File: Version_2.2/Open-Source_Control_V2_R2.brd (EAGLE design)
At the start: 121.9 x 129.5 mm, 344 parts, among them IC10 MCP6002SMT, IC11 MCP6002SMT, IC12 MCP6002SMT, IC14 MCP6002SMT, IC2 ULN2003AD, IC4 74HC165D, IC5 74HC165D, J24 6p-2.54, K1 JS1-24V-F, K2 JS1-24V-F, K3 JS1-24V-F, K4 JS1-24V-F, K5 JS1-24V-F, Q1 MMBT2907, T4 DA2304-AL, U1 OSD3358-512M-ICB, U16 AT97SC3205T-G3M4400B, U2 TPD4S012_DRY_6_P1_M, U27 LAN8710, U28 TCAN1051HV, U29 MAX3483EESA+T, U4 APX811-31UGSOT, U40 ISO3086TDW, U5 TLVH431, U6 SN74LVC2G241_DCU_8, X1 10118194-0001LF, X10 MC4, X11 MC4, X12 MC4, X2 J0011D01BNL, X21 MC10, X24 MSTBA2, X3 MC4, X4 CTI-JTAG, X41 MSTBA3, X5 DM3CS-SF, X6 6p-2.54, X7 TH-2X10, X8 MC4, Y7 7A-25.000MAAE-T

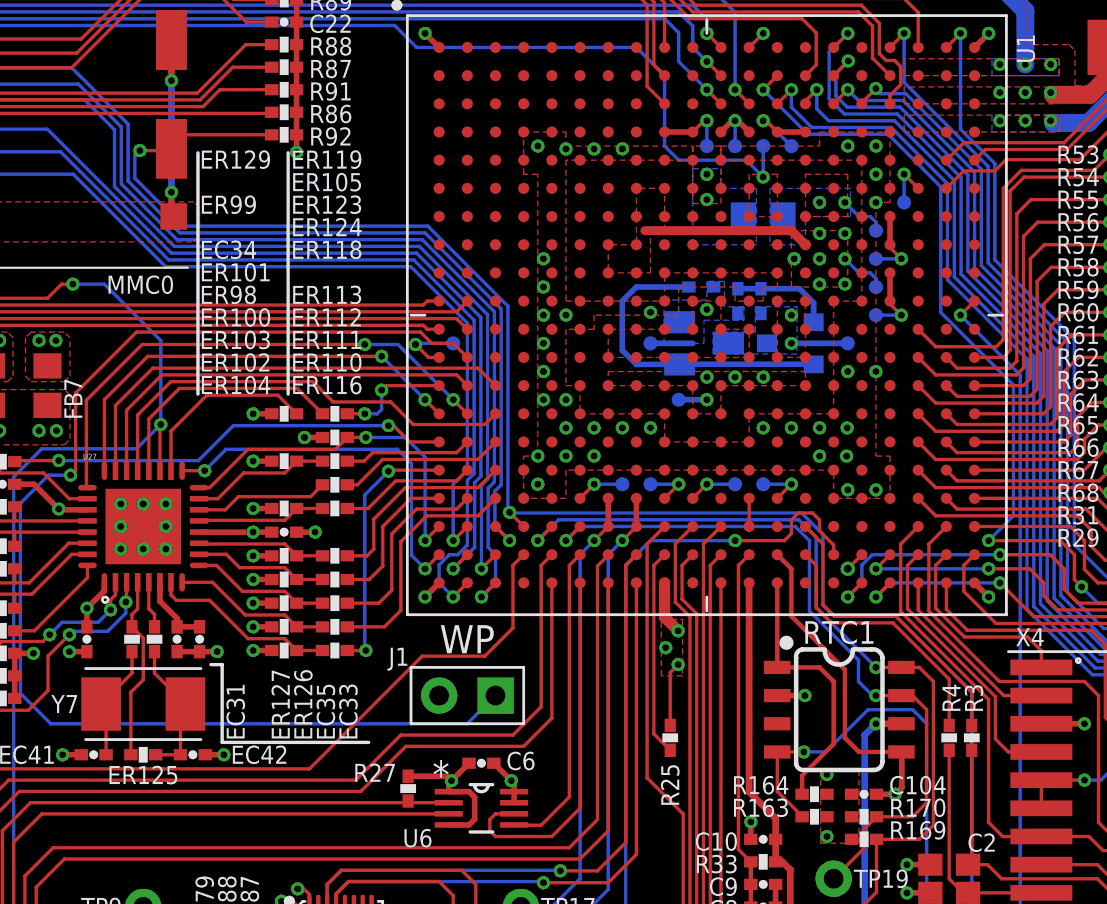
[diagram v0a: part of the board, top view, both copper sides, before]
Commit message: Add files via upload
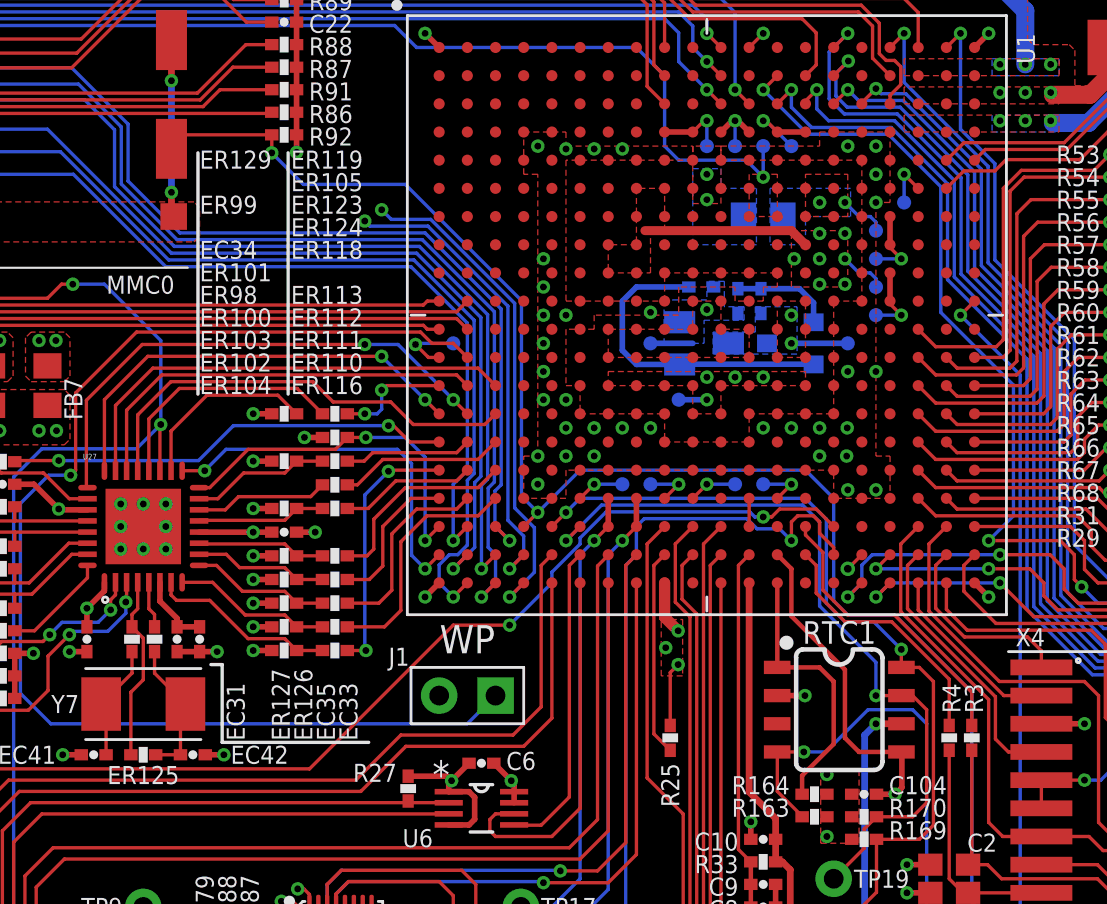
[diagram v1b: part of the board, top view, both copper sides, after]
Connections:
- removed net GPIO0_4: U1.W4, U29.2, U29.3
- new net GPIO0_7: U1.V15, U29.2, U29.3
- new net PR1_PRU0_PRU_R30_6: U1.V17
- new net PR1_PRU0_PRU_R30_7: U1.V16
- new net PR1_UART0_RXD: U1.W4
- new net PR1_UART0_TXD: U1.Y4
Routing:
- net GPIO0_7: track 0.00 -> 49.7 mm, vias 0 -> 4
- net GPIO0_4: track 35.6 -> 0.00 mm, vias 2 -> 0
- net PR1_UART0_TXD: track 0.00 -> 22.7 mm, vias 0 -> 2
- net PR1_UART0_RXD: track 0.00 -> 21.3 mm, vias 0 -> 2
- net MMC0_CD: track 76.0 -> 70.5 mm
- net TPM_GPIO0: track 43.1 -> 44.7 mm
- net I2C1_SDA: track 33.6 -> 35.0 mm
